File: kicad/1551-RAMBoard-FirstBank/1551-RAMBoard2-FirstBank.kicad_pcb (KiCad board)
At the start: 2 copper layers, 58.7 x 40.6 mm, 12 parts, among them J1 Conn_01x02_Male, U1 27C512, U2 74LS139, U3 KM62256CLP, U4_SOCKET1 27128

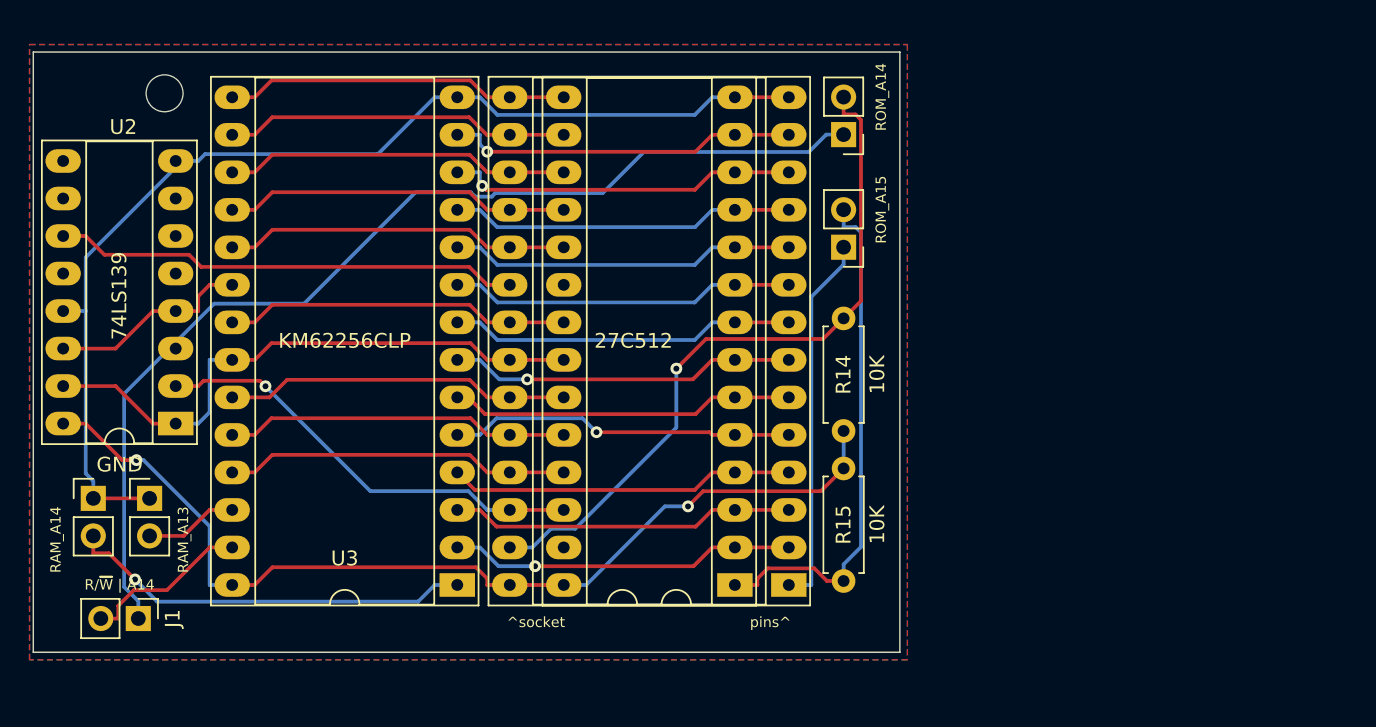
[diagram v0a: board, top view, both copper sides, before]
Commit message: first attempt
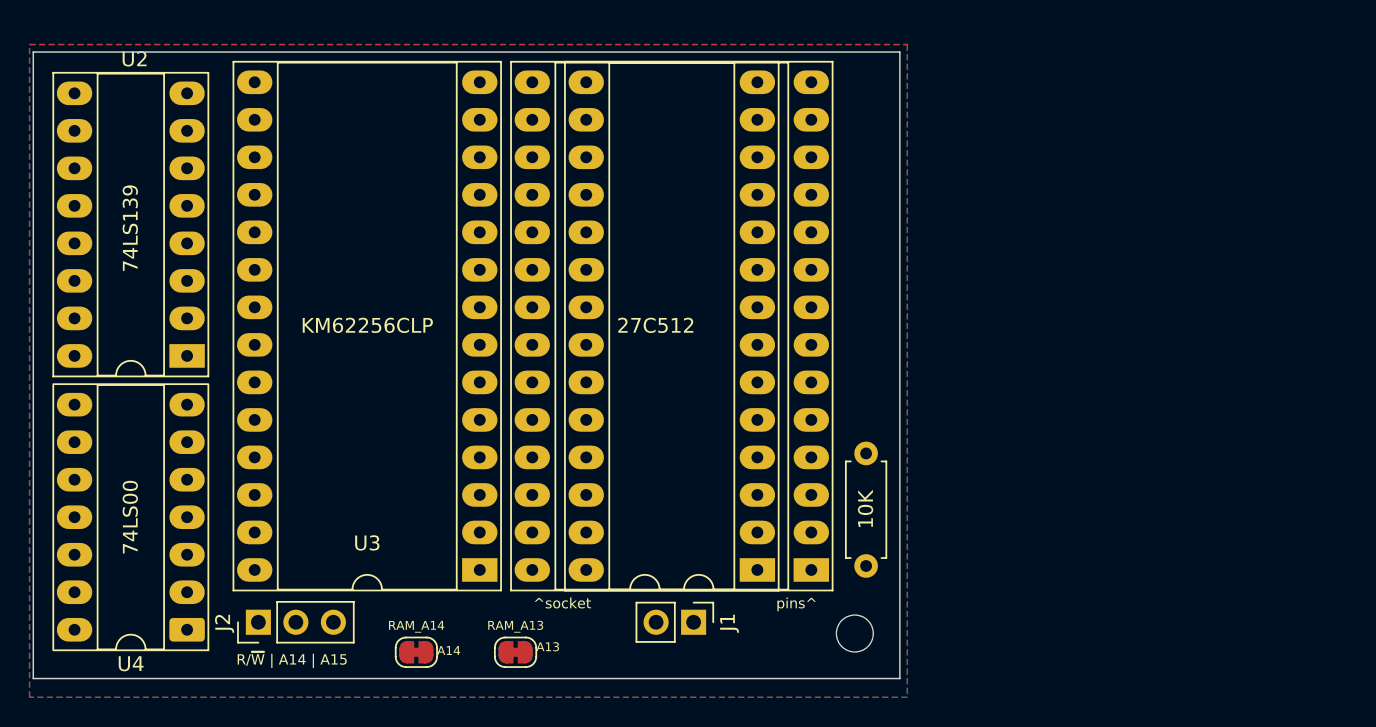
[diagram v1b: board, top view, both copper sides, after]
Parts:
- removed R14: 10K, Resistor_THT:R_Axial_DIN0207_L6.3mm_D2.5mm_P7.62mm_Horizontal
- removed ROM_A14: ROM_A14, Connector_PinHeader_2.54mm:PinHeader_1x02_P2.54mm_Vertical
- removed ROM_A15: ROM_A15, Connector_PinHeader_2.54mm:PinHeader_1x02_P2.54mm_Vertical
- added J2: Conn_01x03_Pin, Connector_PinHeader_2.54mm:PinHeader_1x03_P2.54mm_Vertical, F.Cu at (124.2, 124.2)
- added U4: 74LS00, Package_DIP:DIP-14_W7.62mm_Socket_LongPads, F.Cu at (119.4, 124.7)
- J1: value Conn_01x02_Male -> Conn_01x02_Pin
- RAM_A13: value RAM_A13 -> SolderJumper_2_Bridged; footprint Connector_PinHeader_2.54mm:PinHeader_1x02_P2.54mm_Vertical -> Jumper:SolderJumper-2_P1.3mm_Bridged_RoundedPad1.0x1.5mm
- RAM_A14: value RAM_A14 -> SolderJumper_2_Bridged; footprint Connector_PinHeader_2.54mm:PinHeader_1x02_P2.54mm_Vertical -> Jumper:SolderJumper-2_P1.3mm_Bridged_RoundedPad1.0x1.5mm
- moved H1 59.3 mm to (164.6, 125.0)
- moved J1 37.6 mm to (153.7, 124.2)
- moved RAM_A13 26.9 mm to (141.6, 126.2)
- moved RAM_A14 24.2 mm to (134.9, 126.2)
- moved U2 4.65 mm to (119.4, 106.2)
- moved R15 1.83 mm to (165.4, 112.8)
- moved U1 1.83 mm to (158.0, 120.7)
- moved U3 1.83 mm to (139.2, 120.7)
- moved U4_SOCKET1 1.83 mm to (161.6, 120.7)
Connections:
- J1 pad 1: /A14 -> Net-(J1-Pin_1)
- J1 pad 2: /R/~{W} -> GND
- R15 pad 2: Net-(R15-Pad2) -> Net-(J1-Pin_1)
- U1 pad 1: Net-(R15-Pad2) -> Net-(J1-Pin_1)
- U1 pad 27: Net-(R14-Pad1) -> /A14
- U4_SOCKET1 pad 22: /~{A15} -> unconnected-(U4_SOCKET1-~{OE}-Pad22)
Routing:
- net GND: track 75.4 -> 0.00 mm
- net /A14: track 72.3 -> 0.00 mm
- net VCC: track 66.8 -> 0.00 mm, vias 2 -> 0
- net Net-(R14-Pad1): track 47.8 -> 0.00 mm, vias 1 -> 0
- net /~{A15}: track 39.7 -> 0.00 mm
- net Net-(R15-Pad2): track 35.0 -> 0.00 mm
- net /~{ROMSEL}: track 31.6 -> 0.00 mm
- net /A13: track 30.0 -> 0.00 mm, vias 1 -> 0
- net Net-(RAM_A14-B): track 27.6 -> 0.00 mm, vias 1 -> 0
- net /VPP: track 25.3 -> 0.00 mm
- net /D1: track 23.9 -> 0.00 mm, vias 1 -> 0
- net /D2: track 23.8 -> 0.00 mm, vias 1 -> 0
- net /A3: track 23.5 -> 0.00 mm, vias 1 -> 0
- net /A12: track 23.5 -> 0.00 mm, vias 1 -> 0
- net /A2: track 23.4 -> 0.00 mm
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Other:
- board size 58.7 x 40.6 mm -> 58.7 x 42.4 mm
- board text added: "1551-RAMBOard][ v1.0 (c) XII 2025 Maciej Witkowiak, <ytm@elysium.pl>"
- board text added: "A13"
- board text added: "A14"
- board text added: "J1 selects 32K half of 64K ROM short: bottom half open: top half"
- board text added: "R/~{W} | A14 | A15"
- board text added: "RAM_A13/14 jumpers closed: GND for 8K opened: connect to ??? to have 8K banks"
- board text removed: "1551-RAMBOard][ v1.1 (c) IV 2024 Maciej Witkowiak, <ytm@elysium.pl>"
- board text removed: "GND"
- board text removed: "R/~{W} | A14"
- board text removed: "RAM_A13/14 jumpers closed: GND for 8K opened: connect to VIA#2 PA to have 8K banks"
- board text removed: "ROM_A14 closed: $A000-$FFFF is ROM, omit R14 open: $C000-$FFFF is ROM, install R14 and switch between round pad and GND ROM_A15 closed: 32K ROM or upper half or 64K ROM, omit R15 open: install R15 and switch between round pad and GND"

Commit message: first try
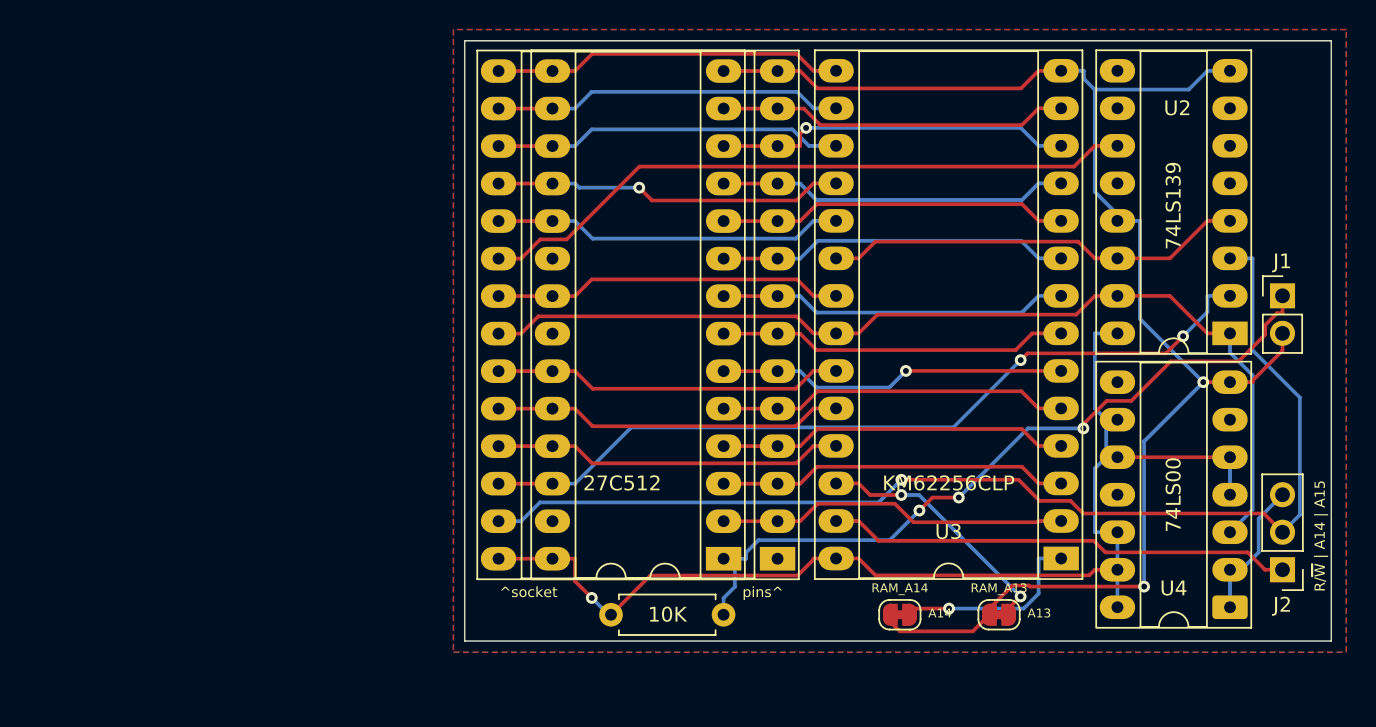
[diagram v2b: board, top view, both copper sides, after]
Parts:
- removed H1: MountingHole, MountingHole:MountingHole_2.5mm
- moved U2 70.6 mm to (190.0, 104.6)
- moved U4 70.6 mm to (190.0, 123.2)
- moved J2 69.4 mm to (193.5, 120.7), turned to 180 degrees
- moved J1 45.6 mm to (193.5, 102.1), turned to 0 degrees
- moved U3 39.4 mm to (178.6, 119.9)
- moved RAM_A13 32.8 mm to (174.4, 123.7)
- moved RAM_A14 32.8 mm to (167.6, 123.7)
- moved R15 20.4 mm to (148.1, 123.7), turned to 0 degrees
- moved U1 2.41 mm to (155.7, 119.9)
- moved U4_SOCKET1 2.41 mm to (159.4, 119.9)
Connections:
- U4_SOCKET1 pad 1: /VPP -> unconnected-(U4_SOCKET1-VPP-Pad1)
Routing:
- net GND: track 0.00 -> 103.0 mm, vias 0 -> 2
- net VCC: track 0.00 -> 80.5 mm, vias 0 -> 1
- net /A14: track 0.00 -> 77.6 mm, vias 0 -> 1
- net /~{A15}: track 0.00 -> 67.3 mm
- net /A13: track 0.00 -> 55.4 mm, vias 0 -> 2
- net Net-(J1-Pin_1): track 0.00 -> 50.8 mm, vias 0 -> 3
- net /~{ROMSEL}: track 0.00 -> 45.1 mm
- net /R/~{W}: track 0.00 -> 31.6 mm
- net /~{RAMSEL}: track 0.00 -> 28.7 mm
- net /D1: track 0.00 -> 24.3 mm, vias 0 -> 1
- net /A12: track 0.00 -> 23.9 mm
- net /A1: track 0.00 -> 23.8 mm
- net /D7: track 0.00 -> 23.8 mm
- net /A11: track 0.00 -> 23.8 mm
- net /A9: track 0.00 -> 23.8 mm
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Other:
- board size 58.7 x 42.4 mm -> 58.7 x 40.6 mm
- board text added: "J1: short: bottom 32K of 64K ROM open: top 32K of 64K ROM"
- board text added: "J2: - A14 from CPU (U2) pin 21 or U7 pin 7 - A15 from CPU (U2) pin 22 or U7 pin 6 - R/~{W} from onboard RAM (U5) pin 21 or or gate array (U6) pin 31(?) or U3 pin 19(?)"
- board text added: "RAM_A13/14 jumpers closed: GND for one 8K bank opened: connect to ??? to select one of four 8K banks"
- board text removed: "J1 A14 from CPU (U3) pin 24 R/~{W} from onboard RAM (U5) pin 21"
- board text removed: "J1 selects 32K half of 64K ROM short: bottom half open: top half"
- board text removed: "RAM_A13/14 jumpers closed: GND for 8K opened: connect to ??? to have 8K banks"
